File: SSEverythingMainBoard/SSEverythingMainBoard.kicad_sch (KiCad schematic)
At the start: 59 parts, among them J1 CONN_06SILK_FEMALE_PTH, J2 CONN_06SILK_FEMALE_PTH, J3 POWER, J4 Switch, J5 Conn_01x02, J6 Conn_01x05, M1 Left MOTOR, M2 Right MOTOR, SW1 TACT_SW, U1 DFRobot_DC_Controller, U3 DC Boost

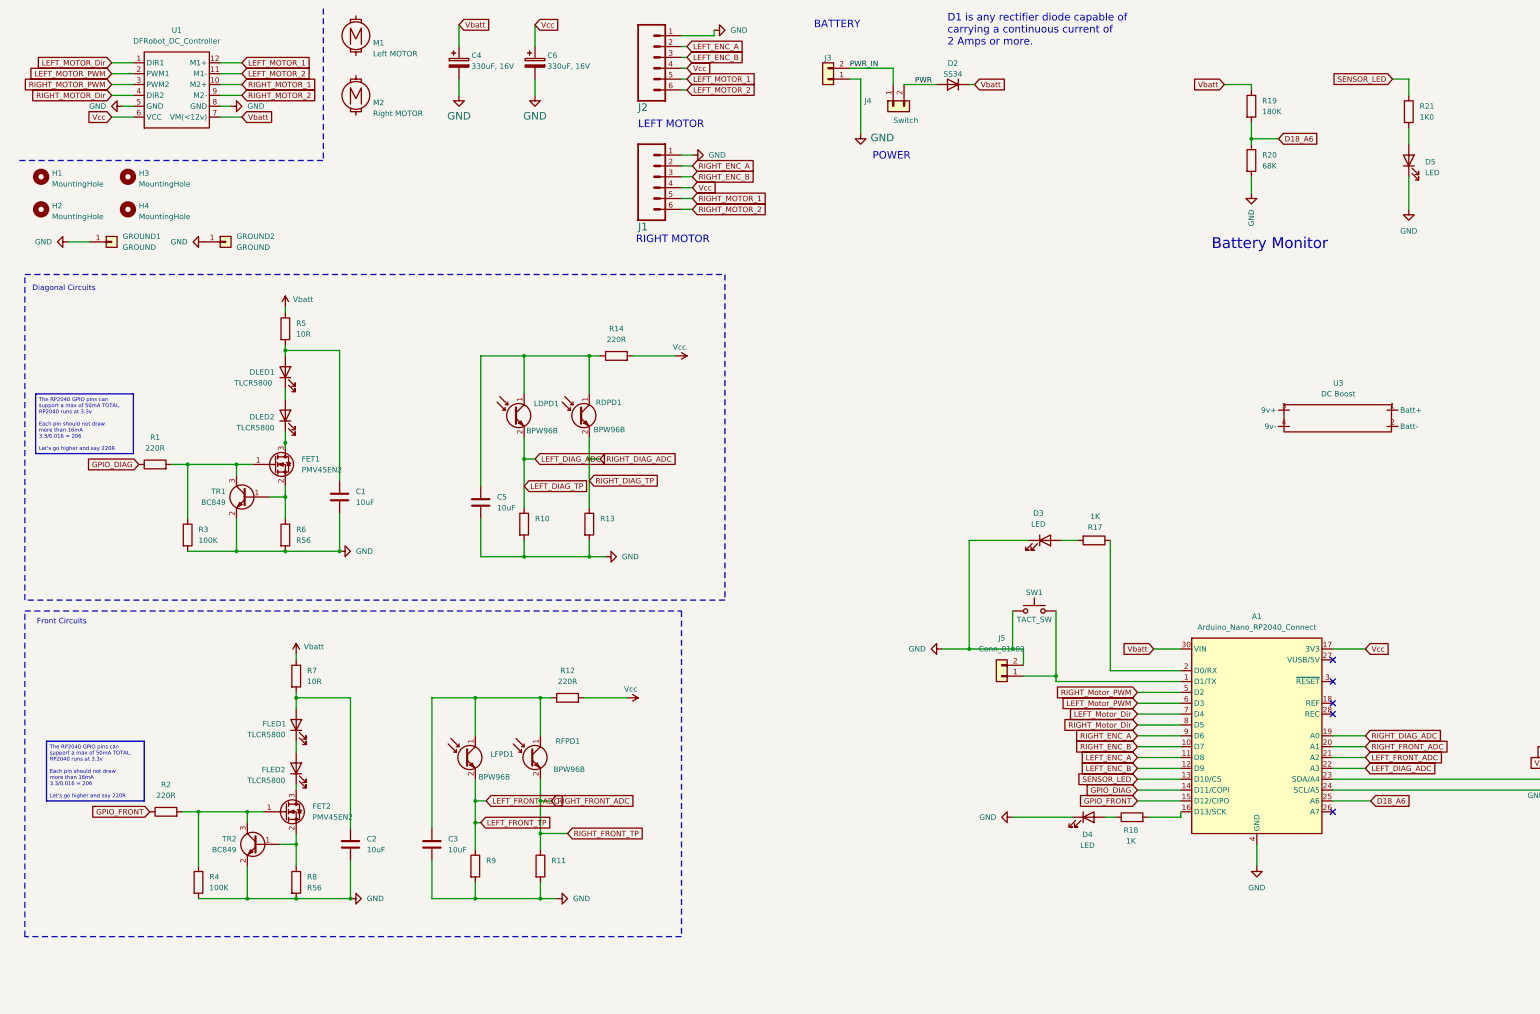
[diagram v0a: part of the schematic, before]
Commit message: Send boards to JLCPCB
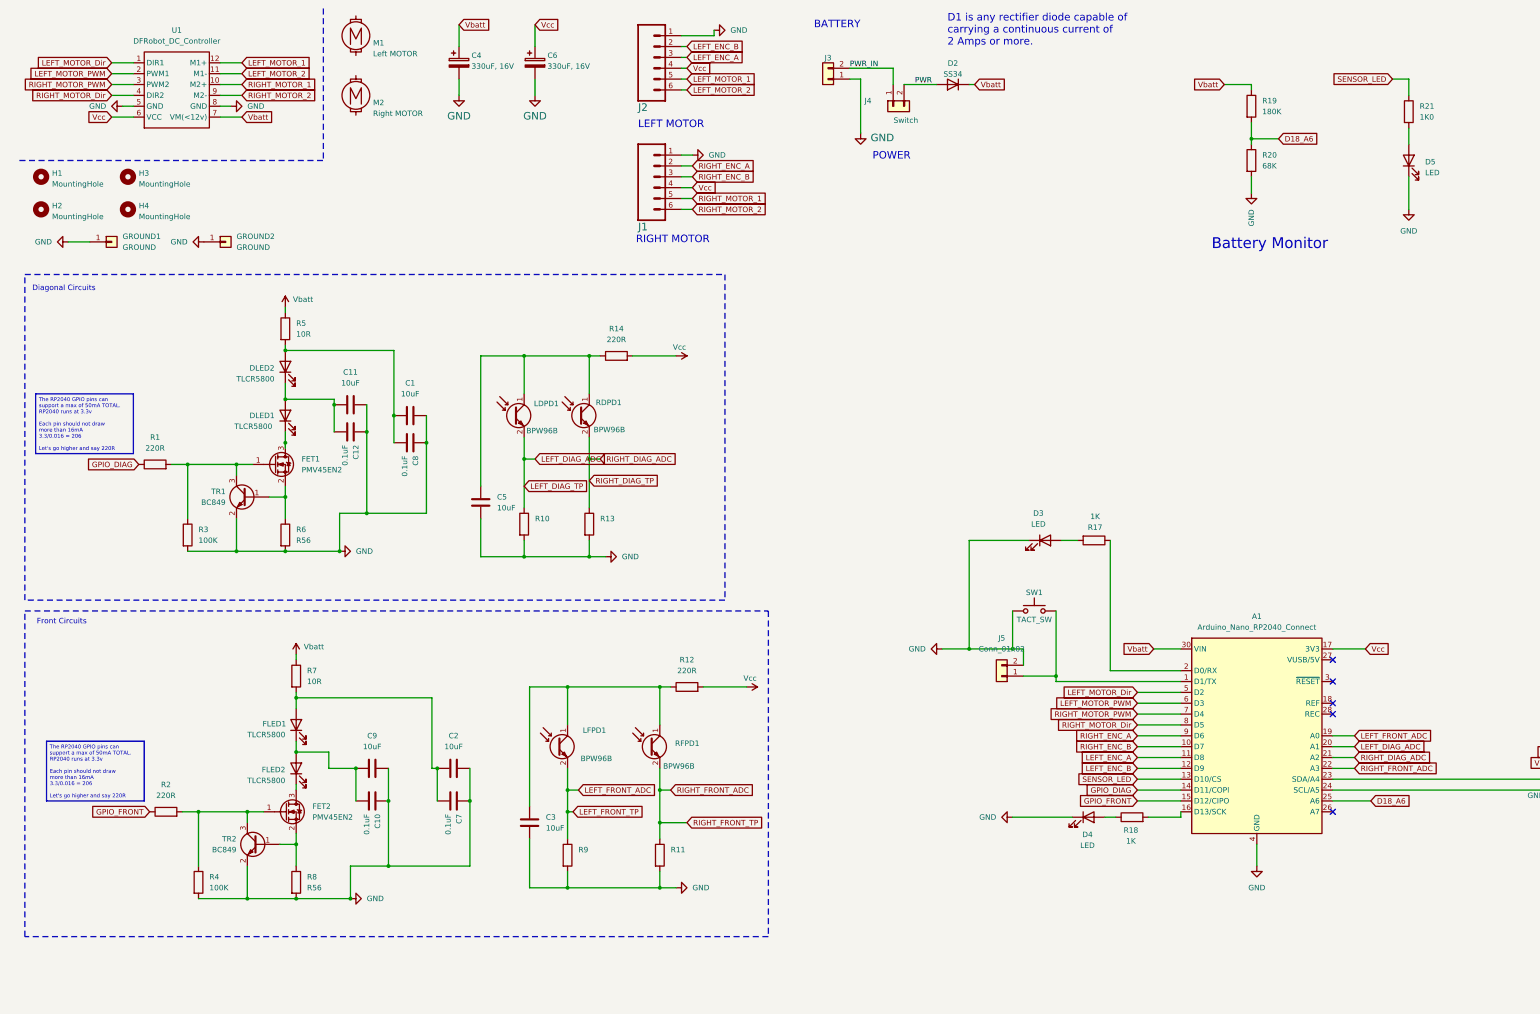
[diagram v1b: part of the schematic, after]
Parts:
- removed U3: DC Boost, symbol Converter_DCDC:DC-DCBoost
- added C10, C12, C7, C8: 0.1uF, Capacitor_SMD:C_0805_2012Metric_Pad1.18x1.45mm_HandSolder, symbol Device:C
- added C11, C9: 10uF, Capacitor_SMD:C_0805_2012Metric_Pad1.18x1.45mm_HandSolder, symbol Device:C
- renumbered RFPD1 to LFPD1, LFPD1 to RFPD1
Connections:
- net LEFT_Motor_Dir is gone; now on net RIGHT_MOTOR_PWM: A1.7 (D4)
- net LEFT_Motor_PWM is gone; now on net LEFT_MOTOR_PWM: A1.6 (D3)
- net RIGHT_Motor_Dir is gone; now on net RIGHT_MOTOR_Dir: A1.8 (D5)
- net RIGHT_Motor_PWM is gone; now on net LEFT_MOTOR_Dir: A1.5 (D2)
- net GND: now also C10.1, C11.2, C12.1, C7.1, C8.1, C9.2
- net LEFT_DIAG_ADC: now also A1.20 (A1); no longer A1.22 (A3)
- net LEFT_ENC_A: now also J2.3; no longer J2.2
- net LEFT_ENC_B: now also J2.2; no longer J2.3
- net LEFT_FRONT_ADC: now also A1.19 (A0), LFPD1.2 (E); no longer A1.21 (A2), RFPD1.2 (E)
- net RIGHT_DIAG_ADC: now also A1.21 (A2); no longer A1.19 (A0)
- net RIGHT_FRONT_ADC: now also A1.22 (A3), RFPD1.2 (E); no longer A1.20 (A1), LFPD1.2 (E)
- net at C2.1, FLED1.2 (A), R7.2: now also C7.2
- net at DLED2.1 (K): now also DLED1.2 (A), C11.1, C12.2; no longer FET1.3 (D)
- net at DLED1.1 (K): now also FET1.3 (D); no longer DLED2.2 (A)
- net at FLED1.1 (K), FLED2.2 (A): now also C10.2, C9.1
- net at C1.1, R5.2: now also DLED2.2 (A), C8.2; no longer DLED1.2 (A)
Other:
- moved on the sheet: C1, C2, C3, DLED1, DLED2, LFPD1, R11, R12, R9, RFPD1
